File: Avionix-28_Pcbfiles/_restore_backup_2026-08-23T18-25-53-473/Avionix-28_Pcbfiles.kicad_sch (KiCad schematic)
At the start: 13 parts, among them J1 Conn_01x02_Pin, J2 Conn_01x02_Pin, U1 TPS54202DDCR

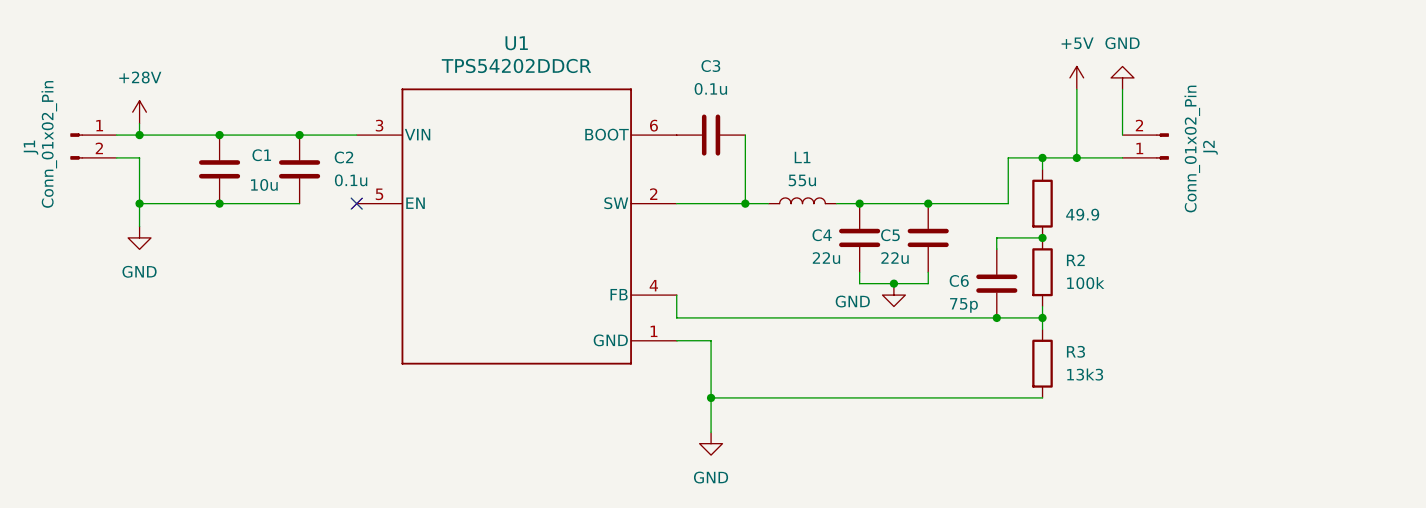
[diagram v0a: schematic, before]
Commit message: base bom
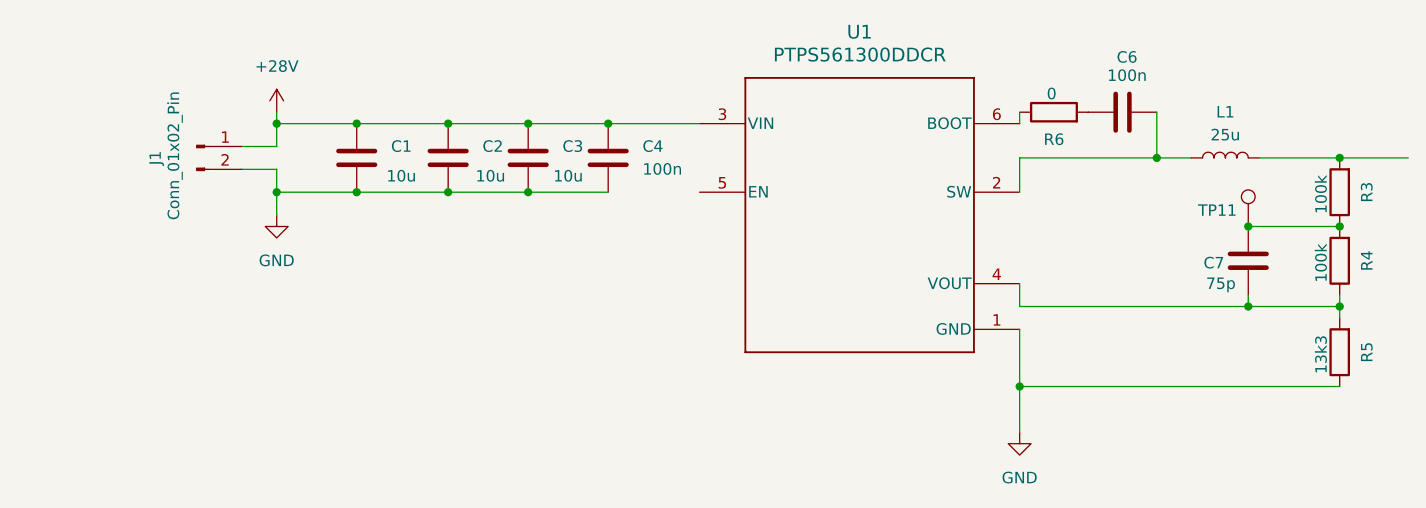
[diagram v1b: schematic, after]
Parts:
- removed C5: 22u, symbol Device:C
- removed J2: Conn_01x02_Pin, Avionix_fprints:CUI_TB007-508-02BE, symbol Connector:Conn_01x02_Pin
- removed R1: 49.9, symbol Device:R
- removed R2: 100k, symbol Device:R
- removed U1: TPS54202DDCR, DDC0006A_N, symbol Avionix-28_symbols:TPS54202DDCR
- added C7: 75p, symbol Device:C
- added R4: 100k, symbol Device:R
- added R5: 13k3, symbol Device:R
- added R6: 0, symbol Device:R
- added TP11: TestPoint, symbol Connector:TestPoint
- added U1: PTPS561300DDCR, DDC0006A-IPC_A, symbol Avionix-28_symbols:PTPS561300DDCR
- C2, C3: value 0.1u -> 10u
- C4: value 22u -> 100n
- C6: value 75p -> 100n
- L1: value 55u -> 25u
- R3: value 13k3 -> 100k
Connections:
- net +28V: now also C3.1, C4.1, U1.3 (VIN)
- net GND: now also C3.2, C4.2, R5.1, U1.1 (GND); no longer C4.1, R3.2
- net at R3.1: now also C7.2, R4.2, TP11.1; no longer C6.1
- net at L1.1: now also C6.2, U1.2 (SW); no longer C3.2
- net +5V: no longer names the net of L1.2
- net +5V: now also R3.2; no longer C4.2
- new net: C7.1, R4.1, R5.2, U1.4 (VOUT)
- new net: R6.1, U1.6 (BOOT)
- new net: C6.1, R6.2
- no-connect marks 1 -> 0
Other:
- moved on the sheet: J1
